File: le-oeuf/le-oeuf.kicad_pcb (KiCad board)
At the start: 2 copper layers, 215.1 x 85 mm, 108 parts, among them J1 Battery JST, J2 Battery, J3 TC2030_SWD, J4 SWD, J5 USB-C Conn, Q1 AO3407, SW1 PG1425, SW10 PG1425, SW11 PG1425, SW12 PG1425, SW13 PG1425, SW14 PG1425, SW15 PG1425, SW16 PG1425, SW17 PG1425, SW18 PG1425, SW19 PG1425, SW2 PG1425, SW20 PG1425, SW21 PG1425, SW22 PG1425, SW23 PG1425, SW24 PG1425, SW25 PG1425, SW26 PG1425, SW27 PG1425, SW28 PG1425, SW29 PG1425, SW3 PG1425, SW30 PG1425, SW31 PG1425, SW32 PG1425, SW33 PG1425, SW34 PG1425, SW35 PG1425, SW36 PG1425, SW4 PG1425, SW5 PG1425, SW6 PG1425, SW7 PG1425, SW8 PG1425, SW9 PG1425, U1 E73-2G4M08S1C-52840, U2 USBLC6-2SC6, U3 TP4054, X1 32.768kHz

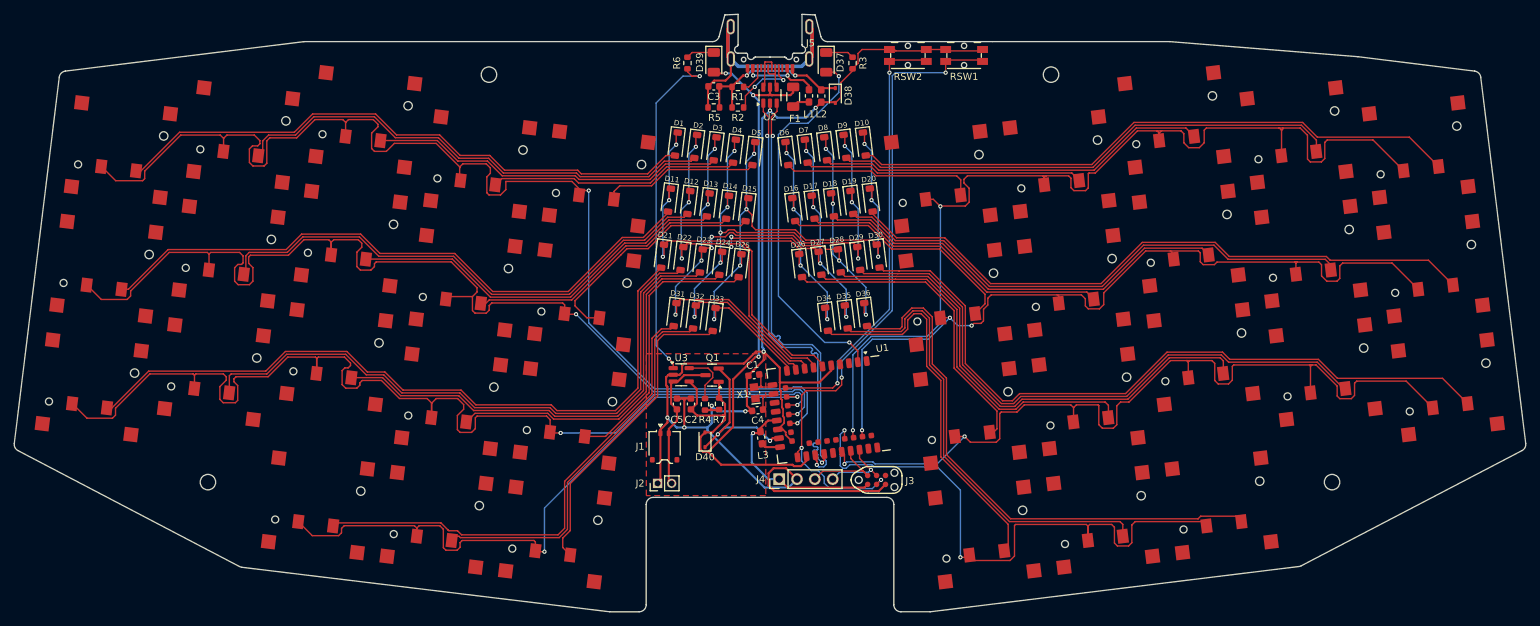
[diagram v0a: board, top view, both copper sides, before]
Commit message: import art
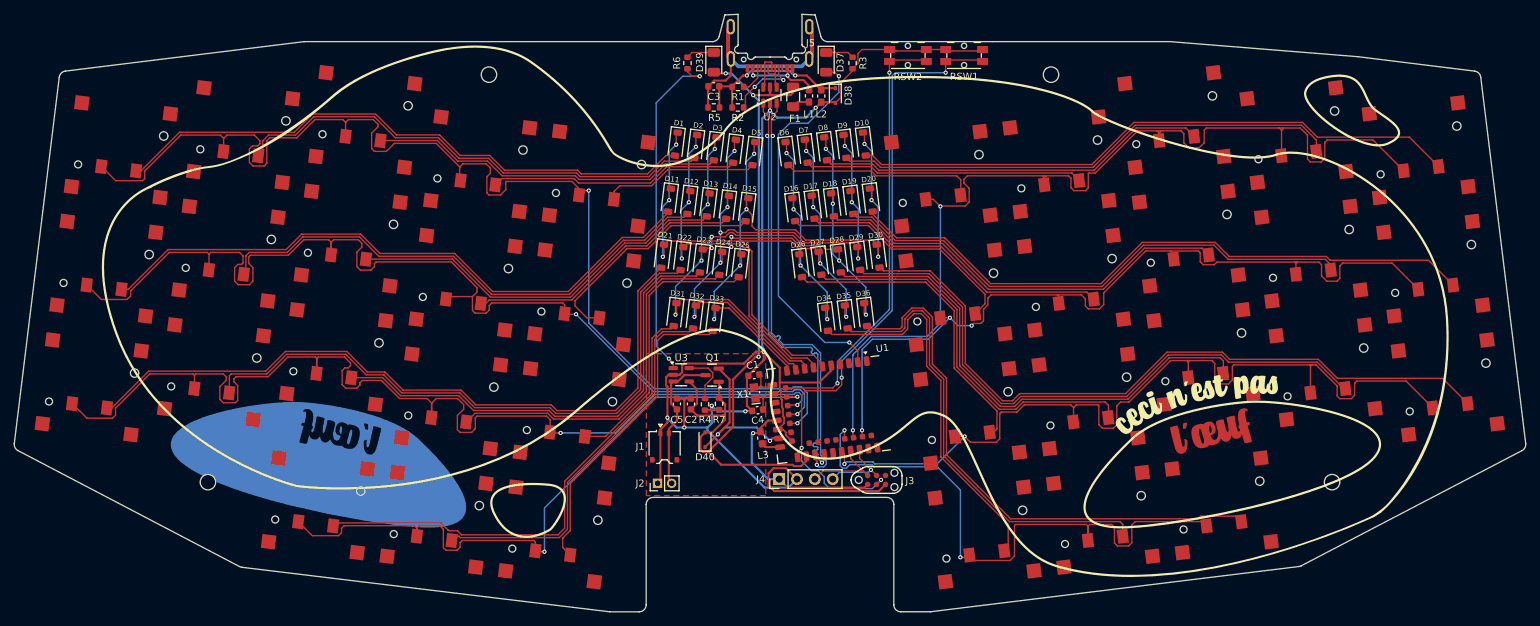
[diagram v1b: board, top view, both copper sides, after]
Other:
- board text added: "art by transthropology"
